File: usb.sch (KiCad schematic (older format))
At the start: 13 parts, among them IC2 AM335X_ZCZ, U6 TPD4S012, U7 TPD4S012, U8 TPS2065CDGN

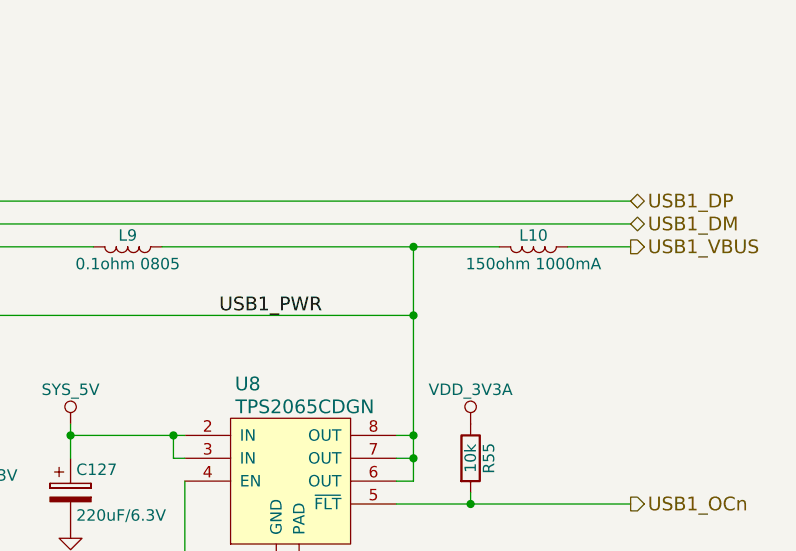
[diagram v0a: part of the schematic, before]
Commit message: erc passed, sch first version
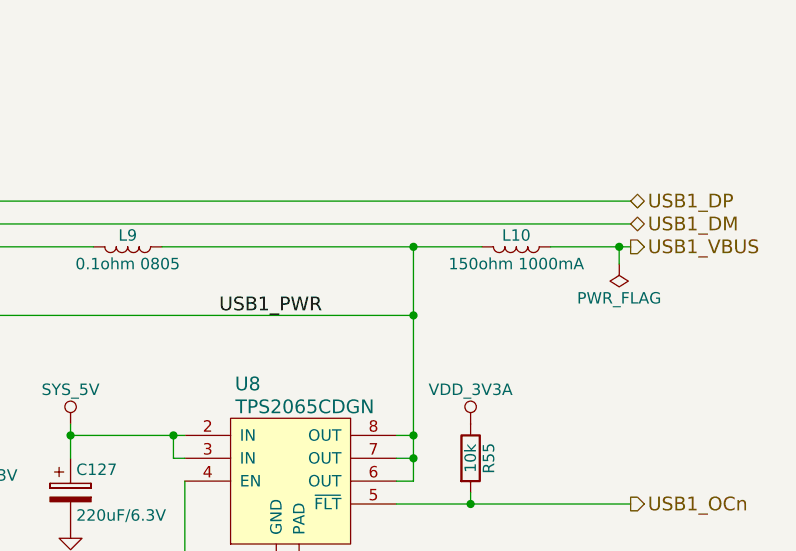
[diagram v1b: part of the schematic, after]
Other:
- moved on the sheet: L10
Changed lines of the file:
@@
 	3800 2350 6025 2350
 $Comp
-L USB_DC #PWR253
+L USB_DC #PWR0269
 U 1 1 58ACAA5E
 P 4900 3450
-F 0 "#PWR253" H 4900 3300 50  0001 C CNN
+F 0 "#PWR0269" H 4900 3300 50  0001 C CNN
 F 1 "USB_DC" H 4900 3600 50  0000 C CNN
 F 2 "" H 4900 3450 50  0000 C CNN
@@
 Connection ~ 4900 3500
 $Comp
-L GNDD #PWR250
+L GNDD #PWR0270
 U 1 1 58ACAB63
 P 4400 4425
-F 0 "#PWR250" H 4400 4175 50  0001 C CNN
+F 0 "#PWR0270" H 4400 4175 50  0001 C CNN
 F 1 "GNDD" H 4400 4275 50  0000 C CNN
 F 2 "" H 4400 4425 50  0000 C CNN
@@
 $EndComp
 $Comp
-L USB_DC #PWR251
+L USB_DC #PWR0271
 U 1 1 58ACAD7C
 P 4825 2250
-F 0 "#PWR251" H 4825 2100 50  0001 C CNN
+F 0 "#PWR0271" H 4825 2100 50  0001 C CNN
 F 1 "USB_DC" V 4825 2500 50  0000 C CNN
 F 2 "" H 4825 2250 50  0000 C CNN
@@
 	6200 3250 6200 3700
 $Comp
-L GNDD #PWR254
+L GNDD #PWR0272
 U 1 1 58ACB114
 P 5700 4425
-F 0 "#PWR254" H 5700 4175 50  0001 C CNN
+F 0 "#PWR0272" H 5700 4175 50  0001 C CNN
 F 1 "GNDD" H 5700 4275 50  0000 C CNN
 F 2 "" H 5700 4425 50  0000 C CNN
@@
 	4525 3050 3800 3050
 $Comp
-L GNDD #PWR252
+L GNDD #PWR0273
 U 1 1 58ACB72B
 P 4825 3050
-F 0 "#PWR252" H 4825 2800 50  0001 C CNN
+F 0 "#PWR0273" H 4825 2800 50  0001 C CNN
 F 1 "GNDD" V 4825 2850 50  0000 C CNN
 F 2 "" H 4825 3050 50  0000 C CNN
@@
 L L L10
 U 1 1 58ACC1B4
-P 8875 2950
-F 0 "L10" V 8825 2950 50  0000 C CNN
-F 1 "150ohm 1000mA" V 8950 2950 50  0000 C CNN
-F 2 "" H 8875 2950 50  0000 C CNN
-F 3 "" H 8875 2950 50  0000 C CNN
-	1    8875 2950
+P 8800 2950
+F 0 "L10" V 8750 2950 50  0000 C CNN
+F 1 "150ohm 1000mA" V 8875 2950 50  0000 C CNN
+F 2 "" H 8800 2950 50  0000 C CNN
+F 3 "" H 8800 2950 50  0000 C CNN
+	1    8800 2950
 	0    1    1    0
 $EndComp
@@
 USB1_VBUS
 Wire Wire Line
-	9300 2950 9025 2950
-Wire Wire Line
-	7250 2950 8725 2950
+	8950 2950 9300 2950
+Wire Wire Line
+	7250 2950 8650 2950
 Wire Wire Line
 	3800 3150 3925 3150
@@
 Connection ~ 7350 4775
 $Comp
-L GNDD #PWR257
+L GNDD #PWR0274
 U 1 1 58ACC7E4
 P 7350 5125
-F 0 "#PWR257" H 7350 4875 50  0001 C CNN
+F 0 "#PWR0274" H 7350 4875 50  0001 C CNN
 F 1 "GNDD" H 7350 4975 50  0000 C CNN
 F 2 "" H 7350 5125 50  0000 C CNN
@@
 Connection ~ 7300 3775
 $Comp
-L GNDD #PWR256
+L GNDD #PWR0275
 U 1 1 58ACCD7F
 P 6850 4175
-F 0 "#PWR256" H 6850 3925 50  0001 C CNN
+F 0 "#PWR0275" H 6850 3925 50  0001 C CNN
 F 1 "GNDD" H 6850 4025 50  0000 C CNN
 F 2 "" H 6850 4175 50  0000 C CNN
@@
 $EndComp
 $Comp
-L SYS_5V #PWR255
+L SYS_5V #PWR0276
 U 1 1 58ACCF48
 P 6850 3725
-F 0 "#PWR255" H 6850 3575 50  0001 C CNN
+F 0 "#PWR0276" H 6850 3575 50  0001 C CNN
 F 1 "SYS_5V" H 6850 3875 50  0000 C CNN
 F 2 "" H 6850 3725 50  0000 C CNN
@@
 Connection ~ 8350 3775
 $Comp
-L GNDD #PWR258
+L GNDD #PWR0277
 U 1 1 58ACD3E3
 P 7800 4575
-F 0 "#PWR258" H 7800 4325 50  0001 C CNN
+F 0 "#PWR0277" H 7800 4325 50  0001 C CNN
 F 1 "GNDD" H 7800 4425 50  0000 C CNN
 F 2 "" H 7800 4575 50  0000 C CNN
@@
 $EndComp
 $Comp
-L VDD_3V3A #PWR259
+L VDD_3V3A #PWR0278
 U 1 1 58ACD7EC
 P 8600 3725
-F 0 "#PWR259" H 8600 3575 50  0001 C CNN
+F 0 "#PWR0278" H 8600 3575 50  0001 C CNN
 F 1 "VDD_3V3A" H 8600 3875 50  0000 C CNN
 F 2 "" H 8600 3725 50  0000 C CNN
@@
 Text Notes 6625 4475 0    60   ~ 0
 tantalum cap
+$Comp
+L PWR_FLAG #FLG0279
+U 1 1 58C56F63
+P 9250 3025
+F 0 "#FLG0279" H 9250 3100 50  0001 C CNN
+F 1 "PWR_FLAG" H 9250 3175 50  0000 C CNN
+F 2 "" H 9250 3025 50  0001 C CNN
+F 3 "" H 9250 3025 50  0001 C CNN
+	1    9250 3025
+	-1   0    0    1
+$EndComp
+Wire Wire Line
+	9250 3025 9250 2950
+Connection ~ 9250 2950
 $EndSCHEMATC

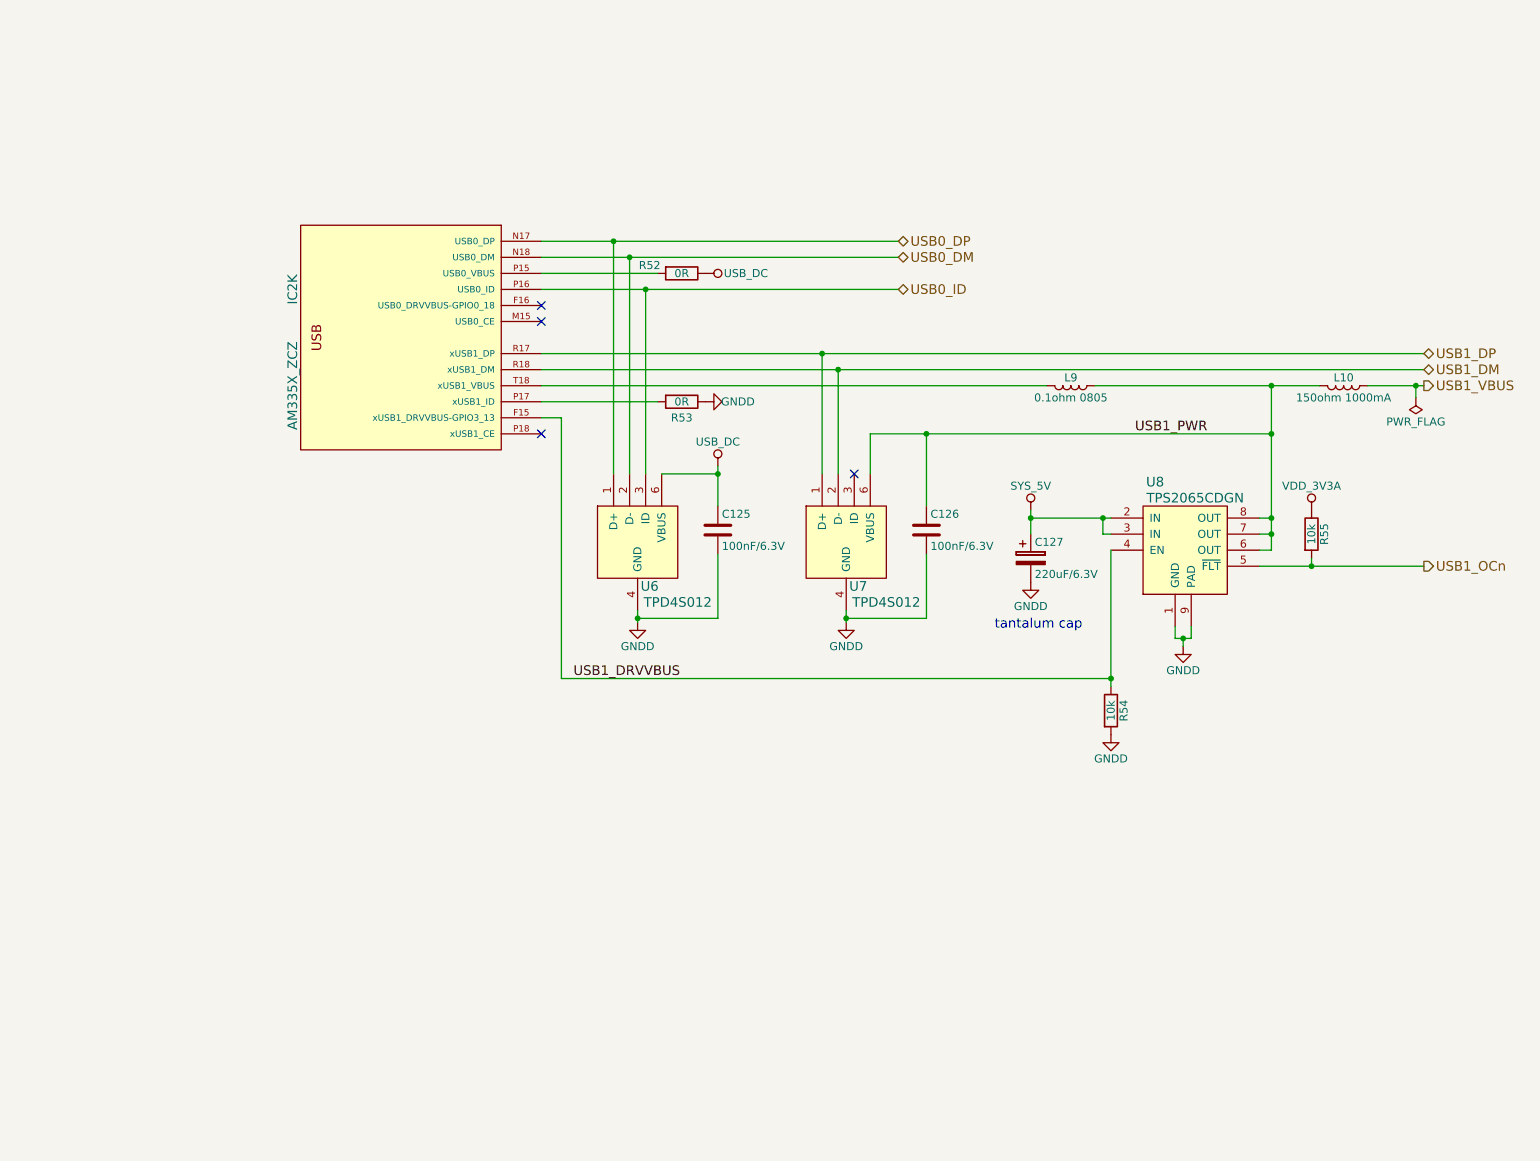
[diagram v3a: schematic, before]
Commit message: wip sys and power
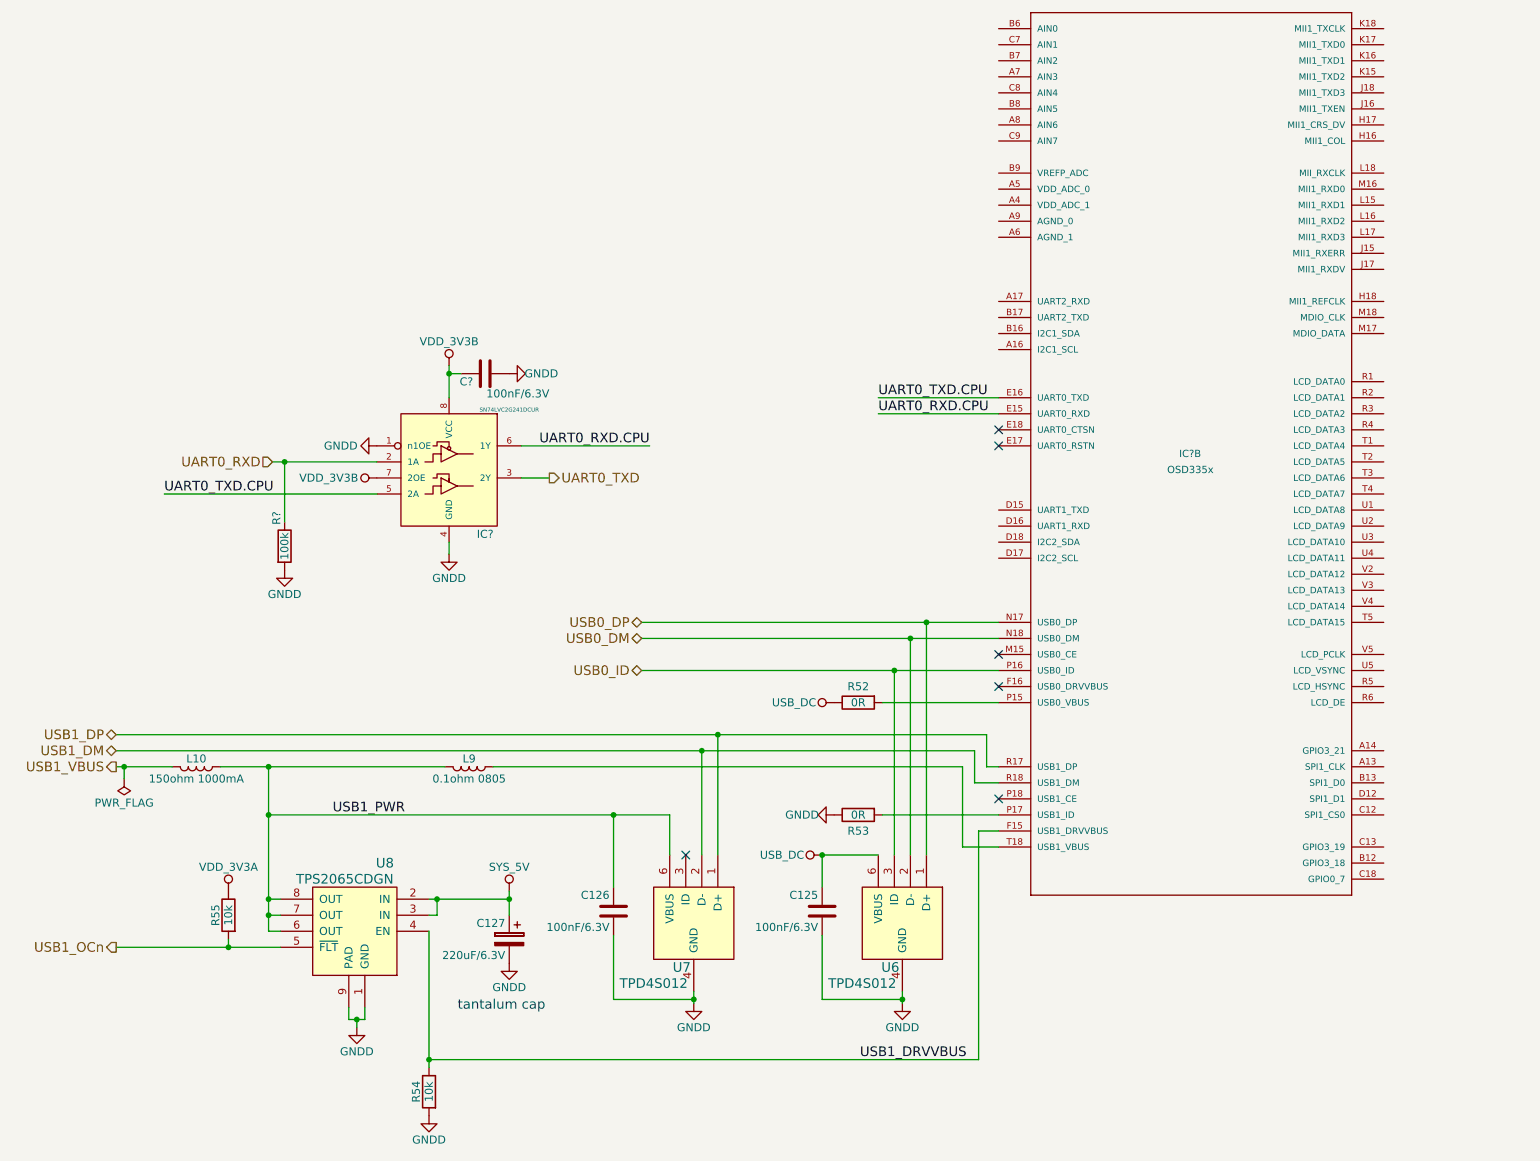
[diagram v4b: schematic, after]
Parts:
- removed IC2: AM335X_ZCZ, footprints:PBGA_N324, symbol AM335X_ZCZ
- added C?: 100nF/6.3V, symbol C
- added IC?: OSD335x, GHI-SoMs-Processors_OSD3358, symbol OSD335x
- added IC?: SN74LVC2G241DCUR, symbol LOGIC-2G125_Dual_3ST_NonInv_Buffer
- added R?: 100k, symbol R
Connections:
- net GNDD: now also C?.2, IC?.1 (n1OE), IC?.4 (GND), R?.2
- net USB0_DM: now also IC?.N18 (USB0_DM)
- net USB0_DP: now also IC?.N17 (USB0_DP)
- net USB0_ID: now also IC?.P16 (USB0_ID)
- net USB1_DM: now also IC?.R18 (USB1_DM)
- net USB1_DP: now also IC?.R17 (USB1_DP)
- net USB1_DRVVBUS: now also IC?.F15 (USB1_DRVVBUS)
- net at R52.2: now also IC?.P15 (USB0_VBUS)
- net at R53.2: now also IC?.P17 (USB1_ID)
- net at L9.2: now also IC?.T18 (USB1_VBUS)
- new net UART0_RXD: IC?.2 (1A), R?.1
- new net UART0_RXD.CPU: IC?.6 (1Y), IC?.E15 (UART0_RXD)
- new net UART0_TXD: IC?.3 (2Y)
- new net UART0_TXD.CPU: IC?.5 (2A), IC?.E16 (UART0_TXD)
- new net VDD_3V3B: C?.1, IC?.7 (2OE), IC?.8 (VCC)
- no-connect marks 4 -> 6
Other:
- moved on the sheet: C125, C126, C127, L10, L9, R52, R53, R54, R55, U6, U7, U8
